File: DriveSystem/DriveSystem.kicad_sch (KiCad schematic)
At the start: 14 parts, among them J1 Raspberry_Pi_2_3, SW1 SW_Push, SW2 SW_Push, SW3 SW_Push, SW4 SW_Push

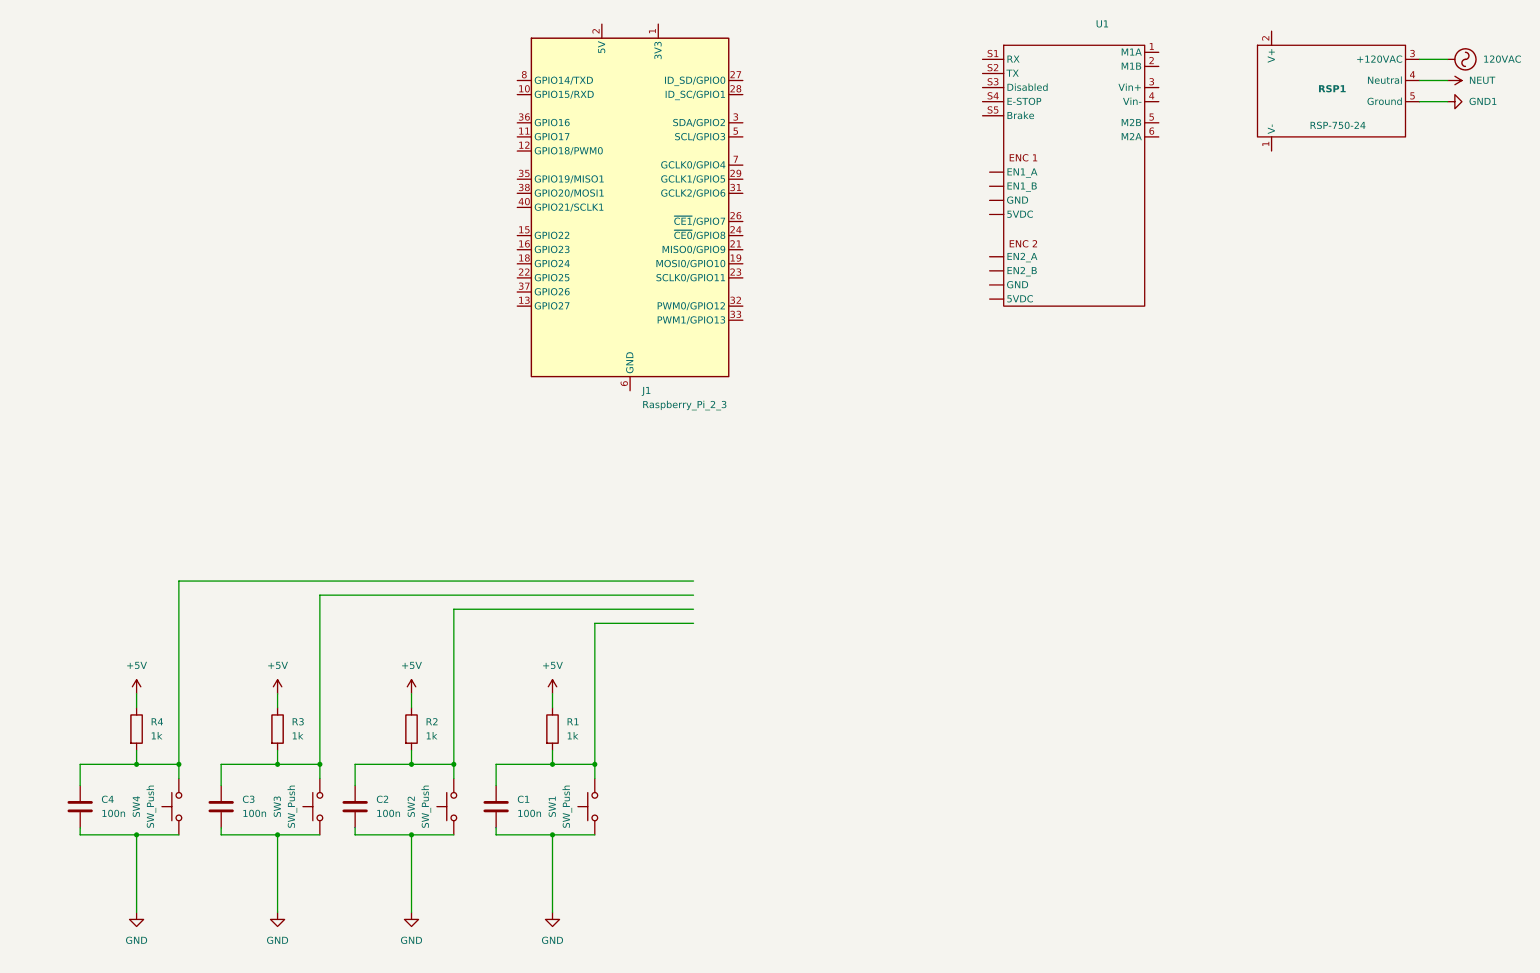
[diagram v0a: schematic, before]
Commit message: Merged RCP Schematic
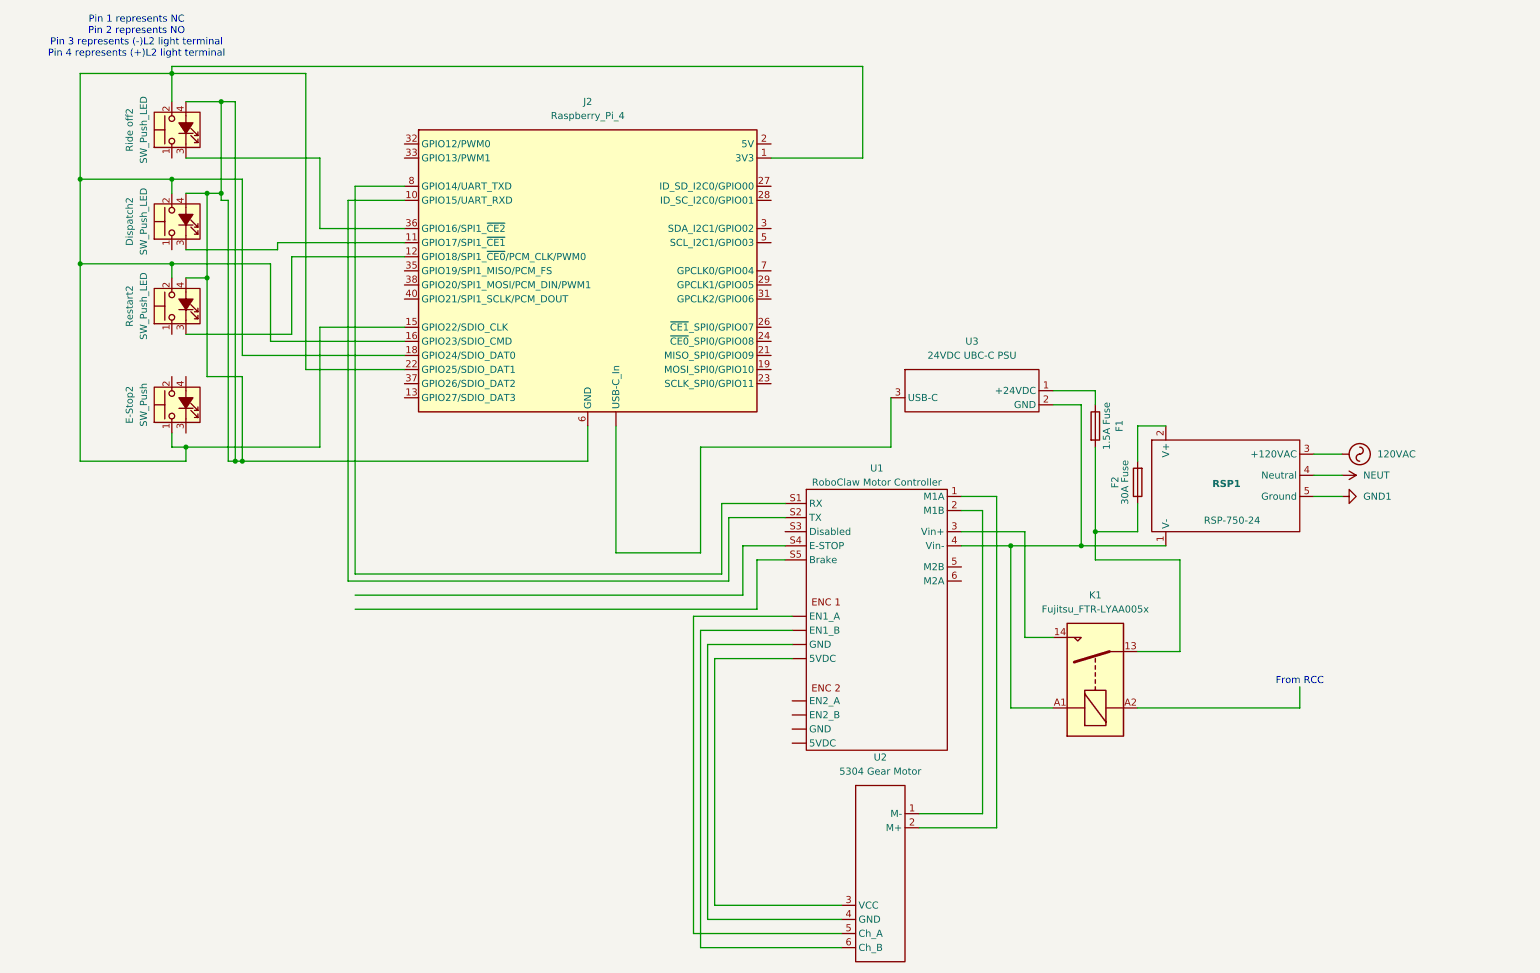
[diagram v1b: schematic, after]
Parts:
- removed C1, C2, C3, C4: 100n, symbol Device:C
- removed J1: Raspberry_Pi_2_3, symbol Connector:Raspberry_Pi_2_3
- removed R1, R2, R3, R4: 1k, symbol Device:R
- removed SW1, SW2, SW3, SW4: SW_Push, symbol Switch:SW_Push
- added Dispatch2, Restart2: SW_Push_LED, symbol Switch:SW_Push_LED
- added E-Stop2: SW_Push, symbol Switch:SW_Push_LED
- added F1: 1.5A Fuse, symbol Device:Fuse
- added F2: 30A Fuse, symbol Device:Fuse
- added J2: Raspberry_Pi_4, symbol Connector:Raspberry_Pi_4
- added K1: Fujitsu_FTR-LYAA005x, Relay_THT:Relay_SPST-NO_Fujitsu_FTR-LYAA005x_FormA_Vertical, symbol Relay:Fujitsu_FTR-LYAA005x
- added Ride off2: SW_Push_LED, symbol Switch:SW_Push_LED
- added U2: 5304 Gear Motor, symbol CustomSymbols:5304_Saturn_Gear_Motor
- added U3: 24VDC UBC-C PSU, symbol CustomSymbols:Pi_PSU
- U1: value ~ -> RoboClaw Motor Controller
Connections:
- net at U1. (5VDC): now also U2.6 (Ch_B)
- net at U1.1 (M1A): now also U2.2 (M+)
- net at U1.2 (M1B): now also U2.1 (M-)
- net at U1.3 (Vin+): now also K1.14
- net at U1.4 (Vin-): now also K1.A1, U3.2 (GND)
- net at U1.S1 (RX): now also J2.8 (GPIO14/UART_TXD)
- net at U1.S2 (TX): now also J2.10 (GPIO15/UART_RXD)
- new net: Dispatch2.2, E-Stop2.1, J2.1 (3V3), J2.15 (GPIO22/SDIO_CLK), J2.16 (GPIO23/SDIO_CMD), J2.17 (3V3), J2.18 (GPIO24/SDIO_DAT0), J2.22 (GPIO25/SDIO_DAT1), Restart2.2, Ride off2.2
- new net: Dispatch2.3 (K), J2.11 (GPIO17/SPI1_~{CE1})
- new net: Dispatch2.4 (A), J2.14 (GND), J2.20 (GND), J2.25 (GND), J2.30 (GND), J2.34 (GND), J2.39 (GND), J2.6 (GND), J2.9 (GND), Restart2.4 (A), Ride off2.4 (A)
- new net: U1. (5VDC), U2.3 (VCC)
- new net: U1. (5VDC), U2.4 (GND)
- new net: U1. (5VDC), U2.5 (Ch_A)
- new net: F1.1, U3.1 (+24VDC)
- new net: F1.2, F2.1, K1.13
- new net: J2. (USB-C_In), U3.3 (USB-C)
- new net: J2.12 (GPIO18/SPI1_~{CE0}/PCM_CLK/PWM0), Restart2.3 (K)
- new net: J2.2 (5V), J2.4 (5V)
- new net: J2.36 (GPIO16/SPI1_~{CE2}), Ride off2.3 (K)
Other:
- note added: "From RCC"
- note added: "Pin 1 represents NC Pin 2 represents NO Pin 3 represents (-)L2 light terminal Pin 4 represents (+)L2 light terminal"
- moved on the sheet: U1
